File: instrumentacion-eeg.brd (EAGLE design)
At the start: 51.7 x 69.8 mm, 39 parts, among them IC1 LMV321AIDCKR, IC15 LMV321AIDCKR, IC16 LMV321AIDCKR, IC2 ESP32-S3-WROOM-1-N4R2, IC3 LMV321AIDCKR, IC5 MCP73831T-2ACI_OT, IC7 AD8226ARZ, IC9 LP38692MP-3.3_NOPB, J1 USB3500-30-A-KIT, J3 SJ-3523-SMT-TR, J4 1769

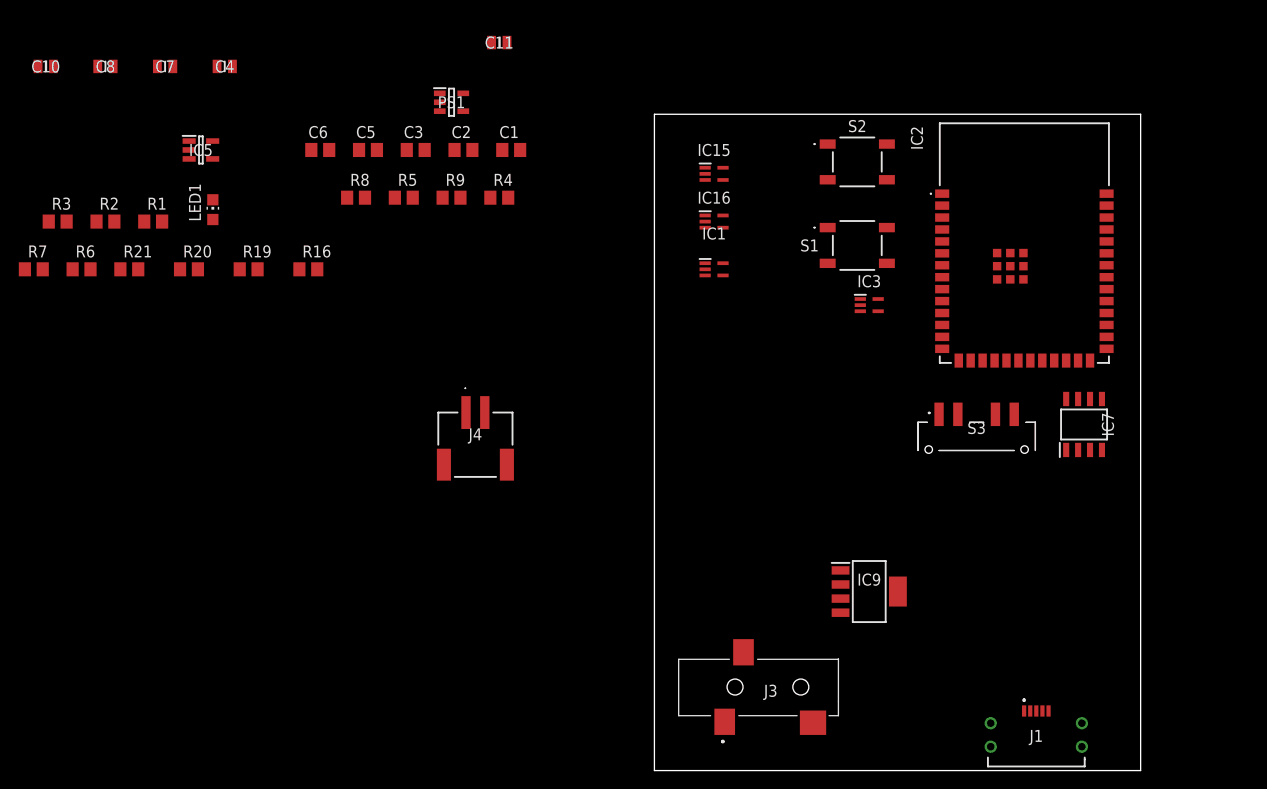
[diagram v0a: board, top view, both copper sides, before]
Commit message: Agrego avance de PCB
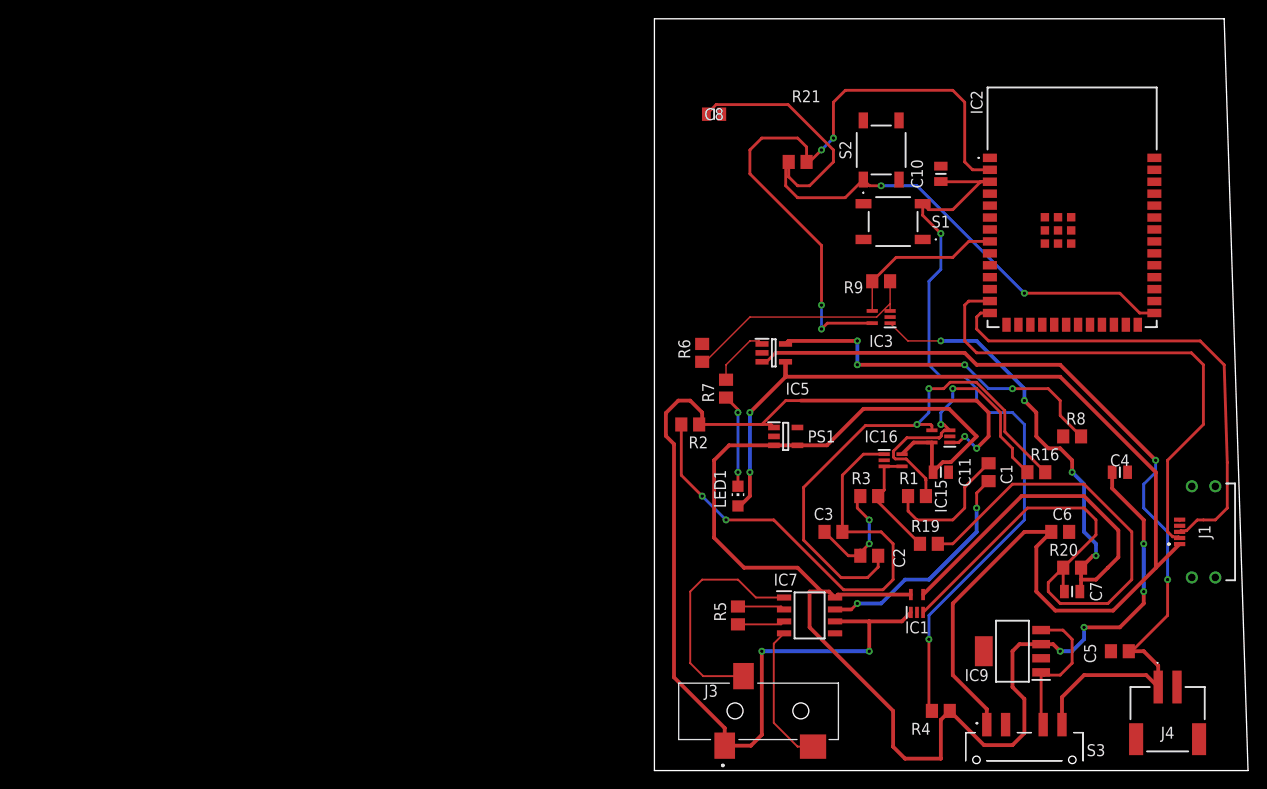
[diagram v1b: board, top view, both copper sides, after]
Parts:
- moved C7 111.5 mm to (44.5, 19.1), turned to 180 degrees
- moved C4 104.6 mm to (49.5, 31.8)
- moved R20 99.2 mm to (44.5, 21.6)
- moved C5 96.2 mm to (49.5, 12.7)
- moved C10 95.9 mm to (30.5, 63.5), turned to 90 degrees
- moved R3 91.2 mm to (22.9, 29.2)
- moved C6 88.6 mm to (43.2, 25.4), turned to 180 degrees
- moved R1 86.4 mm to (27.9, 29.2)
- moved R16 80.4 mm to (40.6, 31.8)
- moved R8 80.3 mm to (44.5, 35.6)
- moved J4 79.2 mm to (54.6, 8.89)
- moved R19 78.1 mm to (29.2, 24.1)
- moved R7 74.7 mm to (7.62, 40.6), turned to 270 degrees
- moved R4 72.0 mm to (30.5, 6.35)
- moved R21 72.0 mm to (15.2, 64.8)
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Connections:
- removed net N$15: IC3.1
- removed net N$7: R6.1
- net N$14: now also R6.1
- net VFOUT: now also IC3.1
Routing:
- net +3V3: track 0.00 -> 230.1 mm, vias 0 -> 8
- net +5V: track 0.00 -> 127.1 mm, vias 0 -> 2
- net VSS: track 0.00 -> 122.7 mm, vias 0 -> 4
- net +BATT: track 0.00 -> 91.2 mm, vias 0 -> 2
- net N$5: track 0.00 -> 80.7 mm, vias 0 -> 2
- net VFOUT: track 0.00 -> 78.0 mm, vias 0 -> 4
- net N$9: track 0.00 -> 76.8 mm
- net N$13: track 0.00 -> 74.4 mm, vias 0 -> 2
- net N$47: track 0.00 -> 56.1 mm, vias 0 -> 2
- net N$3: track 0.00 -> 54.6 mm, vias 0 -> 2
- net -D: track 0.00 -> 54.0 mm
- net +D: track 0.00 -> 52.1 mm
- net N$17: track 0.00 -> 38.2 mm, vias 0 -> 4
- net N$46: track 0.00 -> 33.2 mm, vias 0 -> 2
- net N$14: track 0.00 -> 25.7 mm
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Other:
- board size 51.7 x 69.8 mm -> 63.2 x 80 mm
